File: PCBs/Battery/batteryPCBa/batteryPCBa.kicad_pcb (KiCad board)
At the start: 2 copper layers, 54.5 x 42 mm, 9 parts, among them J1 ToVSensor, J2 Batt1, J3 ESP32-5V, J4 ToMotors, J5 Batt2, J6 SeriesSwitch

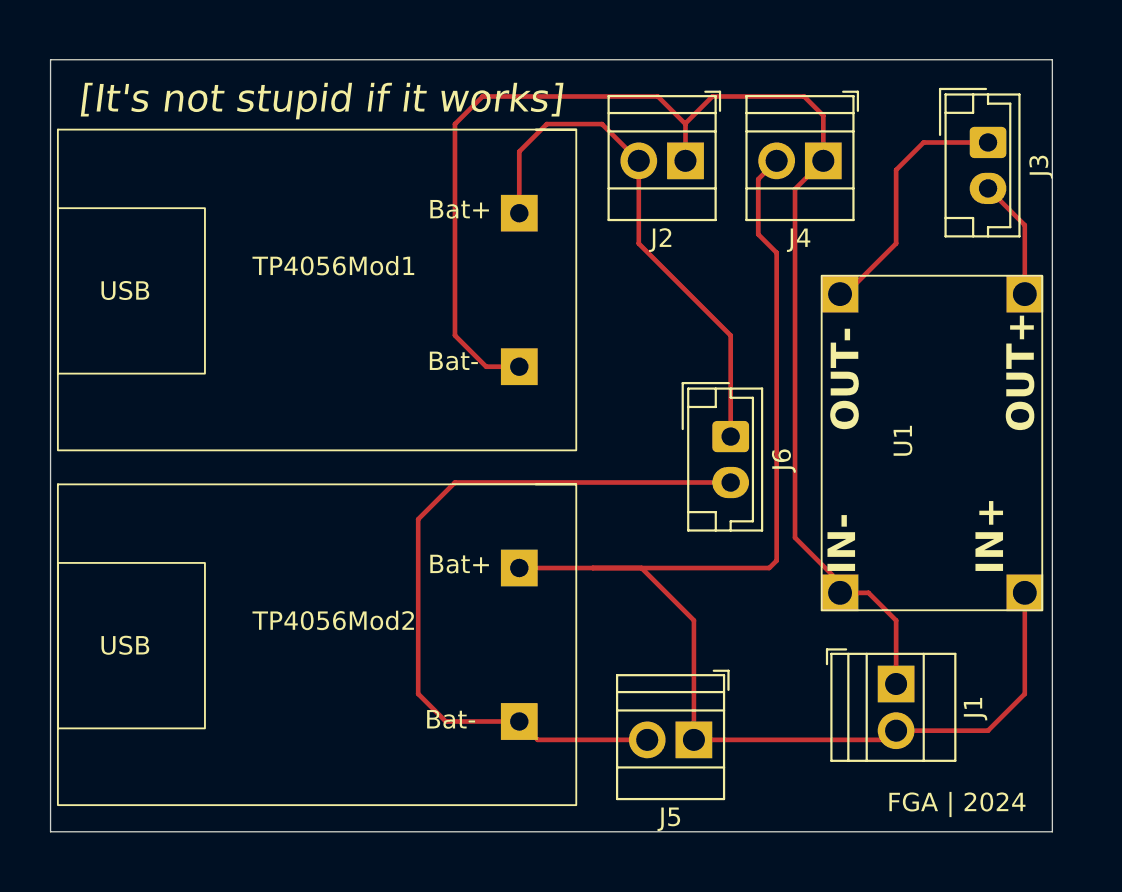
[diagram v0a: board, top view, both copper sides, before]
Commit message: PCBa Ultima
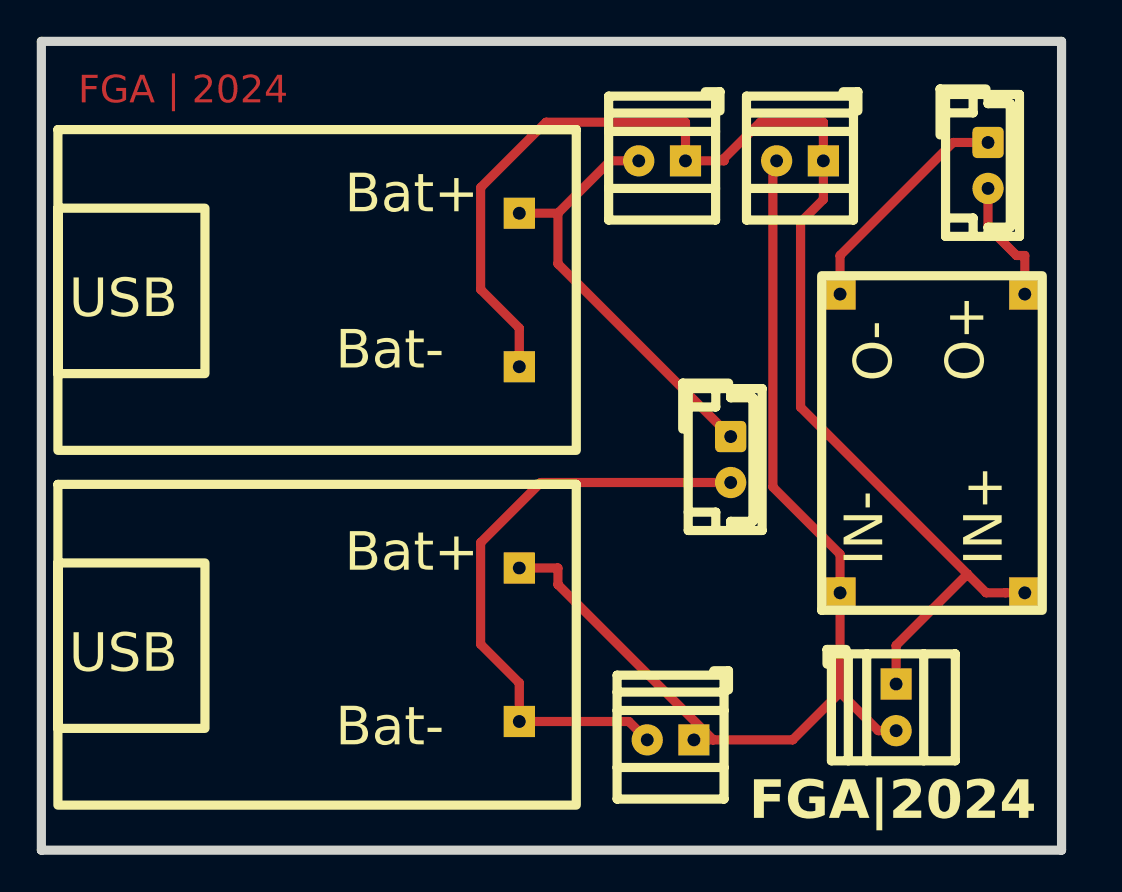
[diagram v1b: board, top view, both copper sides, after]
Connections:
- U1 pad 3: +7.4V -> GND
- U1 pad 4: GND -> +7.4V
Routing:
- net GND: track 74.5 -> 58.4 mm
- net Net-(J5-Pin_2): track 40.8 -> 32.9 mm
- net Net-(J2-Pin_2): track 28.4 -> 23.7 mm
- net +7.4V: track 75.5 -> 73.8 mm
- net Net-(J3-Pin_1): track 13.8 -> 12.7 mm
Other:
- board size 54.5 x 42 mm -> 55.5 x 44 mm
- board text added: "FGA|2024"
- board text removed: "[It's not stupid if it works]"
